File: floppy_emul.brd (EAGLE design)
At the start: 79.7 x 35.5 mm, 33 parts, among them Q1 16MHz, U1 ATMEGA328P, U2 HEF4050B, U3 PCF8574T, U4 LM1117 3.3V

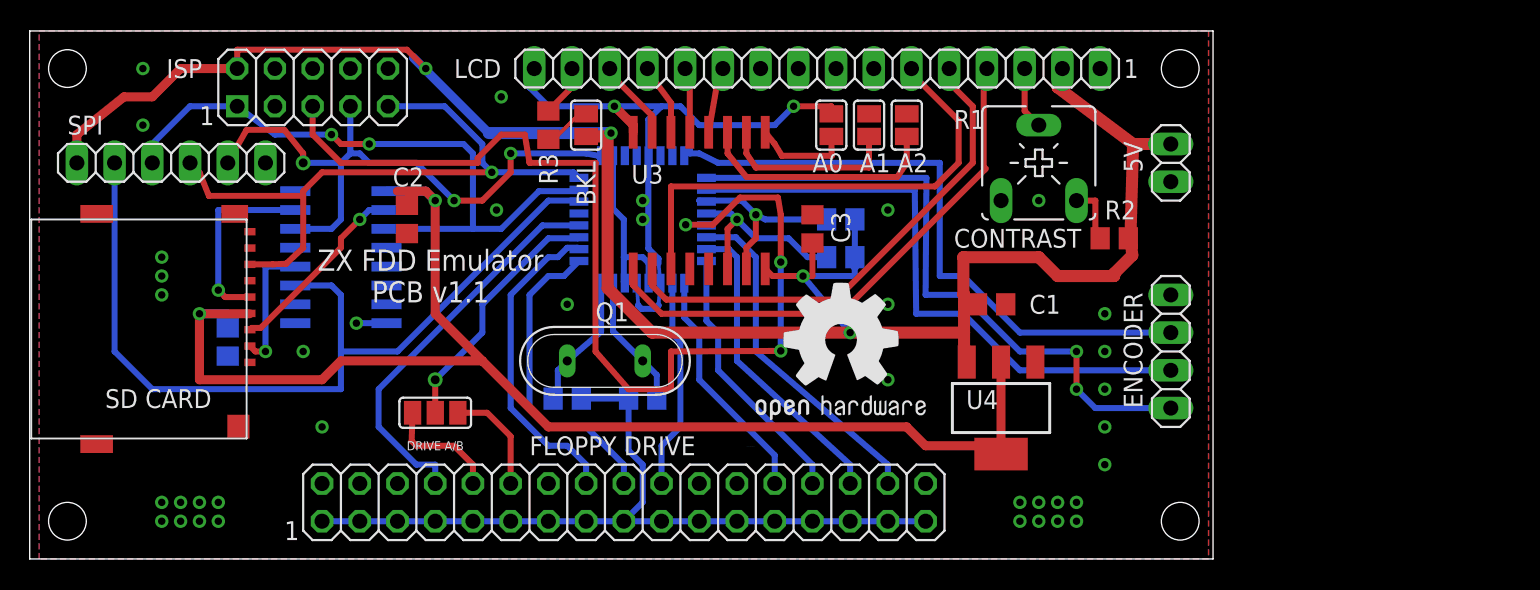
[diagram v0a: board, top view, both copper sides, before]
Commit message: board v1.2
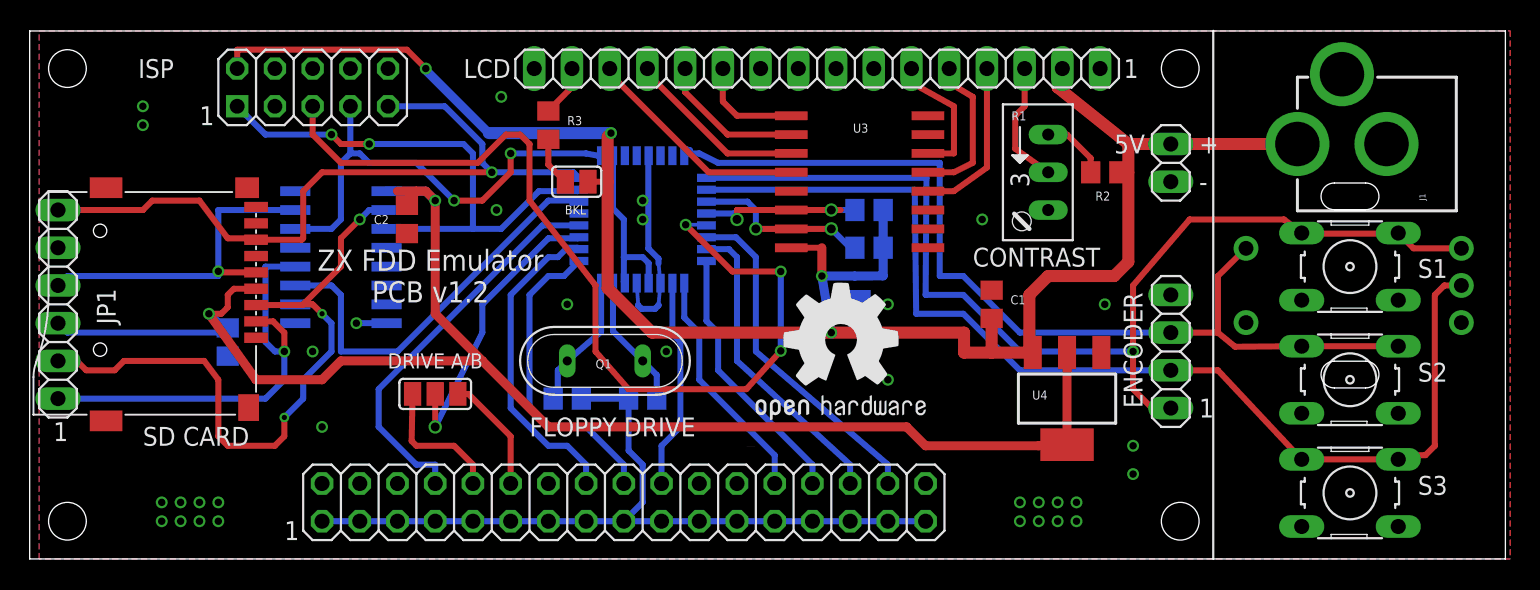
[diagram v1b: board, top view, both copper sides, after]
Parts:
- removed CONN6: MICROSD-PUSH-OUT, microsd:MICROSD-PUSH-OUT
- removed CONN7: SPI, pinhead:1X06
- removed SJ1: A0, jumper:SJ
- removed SJ2: A1, jumper:SJ
- removed SJ3: A2, jumper:SJ
- added J1: POWER_JACKPTH, SparkFun-Connectors:POWER_JACK_PTH
- added JP1: EXT SD CARD, pinhead:1X06
- added S1, S2, S3: (no value), switch-omron:B3F-10XX
- added SD1: ST-TF-003A, Seeed-Connector:MICRO-SD9+4P-SMD-16.1X14.5X1.85MM
- added SW1: ENCODER, piher:CI-11
- R1: device pot:CA6V -> pot:RJ9W
- moved U3 10.9 mm to (55.9, 25.4), turned to 90 degrees
- moved C3 6.54 mm to (55.9, 16.5), flipped to the bottom
- moved R2 4.49 mm to (72.4, 26.0)
- moved U4 4.49 mm to (69.8, 10.8)
- moved SJ4 3.86 mm to (36.8, 25.4), turned to 0 degrees
- moved R4 3.70 mm to (56.5, 23.5)
- moved R5 2.69 mm to (56.5, 21.0)
- moved SJ5 1.27 mm to (27.3, 11.1)
- moved R1 0.64 mm to (67.9, 26.0), turned to 270 degrees
- turned C1 to 90 degrees
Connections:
- removed net N$3: SJ1.2, U3.1
- removed net N$4: SJ2.2, U3.2
- removed net N$5: SJ3.2, U3.3
- new net LCD_LIGHT: U3.7
- net 3V3: now also JP1.3, SD1.4; no longer CONN6.4
- net CLK: no longer CONN7.5
- net ENC_A: now also S1.1, S1.2, SW1.A
- net ENC_B: now also S3.1, S3.2, SW1.B
- net ENC_BTN: now also S2.1, S2.2, SW1.D
- net GND: now also J1.GND, J1.GNDBREAK, JP1.5, S1.3, S1.4, S2.3, S2.4, S3.3, S3.4, SD1.6, SD1.G1, SD1.G2, SD1.G3, SD1.G4, SW1.C, SW1.E, U3.1, U3.2, U3.3; no longer CONN6.6, CONN6.G1, CONN6.G2, CONN6.G3, CONN6.G4, CONN7.6, SJ1.1, SJ2.1, SJ3.1
- net LCD_D4: now also U3.9; no longer U3.4
- net LCD_D5: now also U3.10; no longer U3.5
- net LCD_D6: now also U3.11; no longer U3.6
- net LCD_D7: now also U3.12; no longer U3.7
- net LCD_E: now also U3.6; no longer U3.11
- net LCD_RS: now also U3.4; no longer U3.9
- net LCD_RW: now also U3.5; no longer U3.10
- net MISO: now also JP1.6, SD1.7; no longer CONN6.7, CONN7.4
- net MOSI: no longer CONN7.3
- net SDSEL: no longer CONN7.2
- net SD_CLK: now also JP1.4, SD1.5; no longer CONN6.5
- net SD_MOSI: now also JP1.2, SD1.3; no longer CONN6.3
- net SD_SDSEL: now also JP1.1, SD1.2; no longer CONN6.2
- net VCC: now also J1.PWR; no longer CONN7.1
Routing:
- net ENC_B: track 41.1 -> 74.1 mm
- net SD_MOSI: track 12.9 -> 44.7 mm, vias 1 -> 3
- net SDSEL: track 58.9 -> 27.4 mm
- net ENC_A: track 43.8 -> 73.9 mm, vias 2 -> 1
- net GND: track 98.4 -> 68.7 mm, vias 40 -> 33
- net LCD_RS: track 36.7 -> 11.1 mm
- net LCD_E: track 33.4 -> 9.15 mm
- net LCD_RW: track 34.1 -> 10.4 mm
- net ENC_BTN: track 42.5 -> 64.6 mm
- net SD_SDSEL: track 8.92 -> 29.8 mm
- net N$5: track 16.5 -> 0.00 mm
- net 3V3: track 93.5 -> 107.2 mm
- net N$4: track 12.3 -> 0.00 mm
- net SD_CLK: track 12.9 -> 23.3 mm
- net CLK: track 41.8 -> 31.5 mm, vias 3 -> 2
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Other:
- board size 79.7 x 35.5 mm -> 99.4 x 35.5 mm
- board text added: "+"
- board text added: "-"
- board text added: "ZX FDD Emulator PCB v1.2"
- board text removed: "A0"
- board text removed: "A1"
- board text removed: "A2"
- board text removed: "SPI"
- board text removed: "ZX FDD Emulator PCB v1.1"
